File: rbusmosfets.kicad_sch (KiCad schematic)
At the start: 12 parts, among them J1 RBUS, J4 Conn_01x02_Male, Q4 PXP012-30QLJ, Q5 PXP012-30QLJ, Q6 PXP012-30QLJ, Q7 PXP012-30QLJ, U10 LTC4412xS6, U9 LTC4412xS6

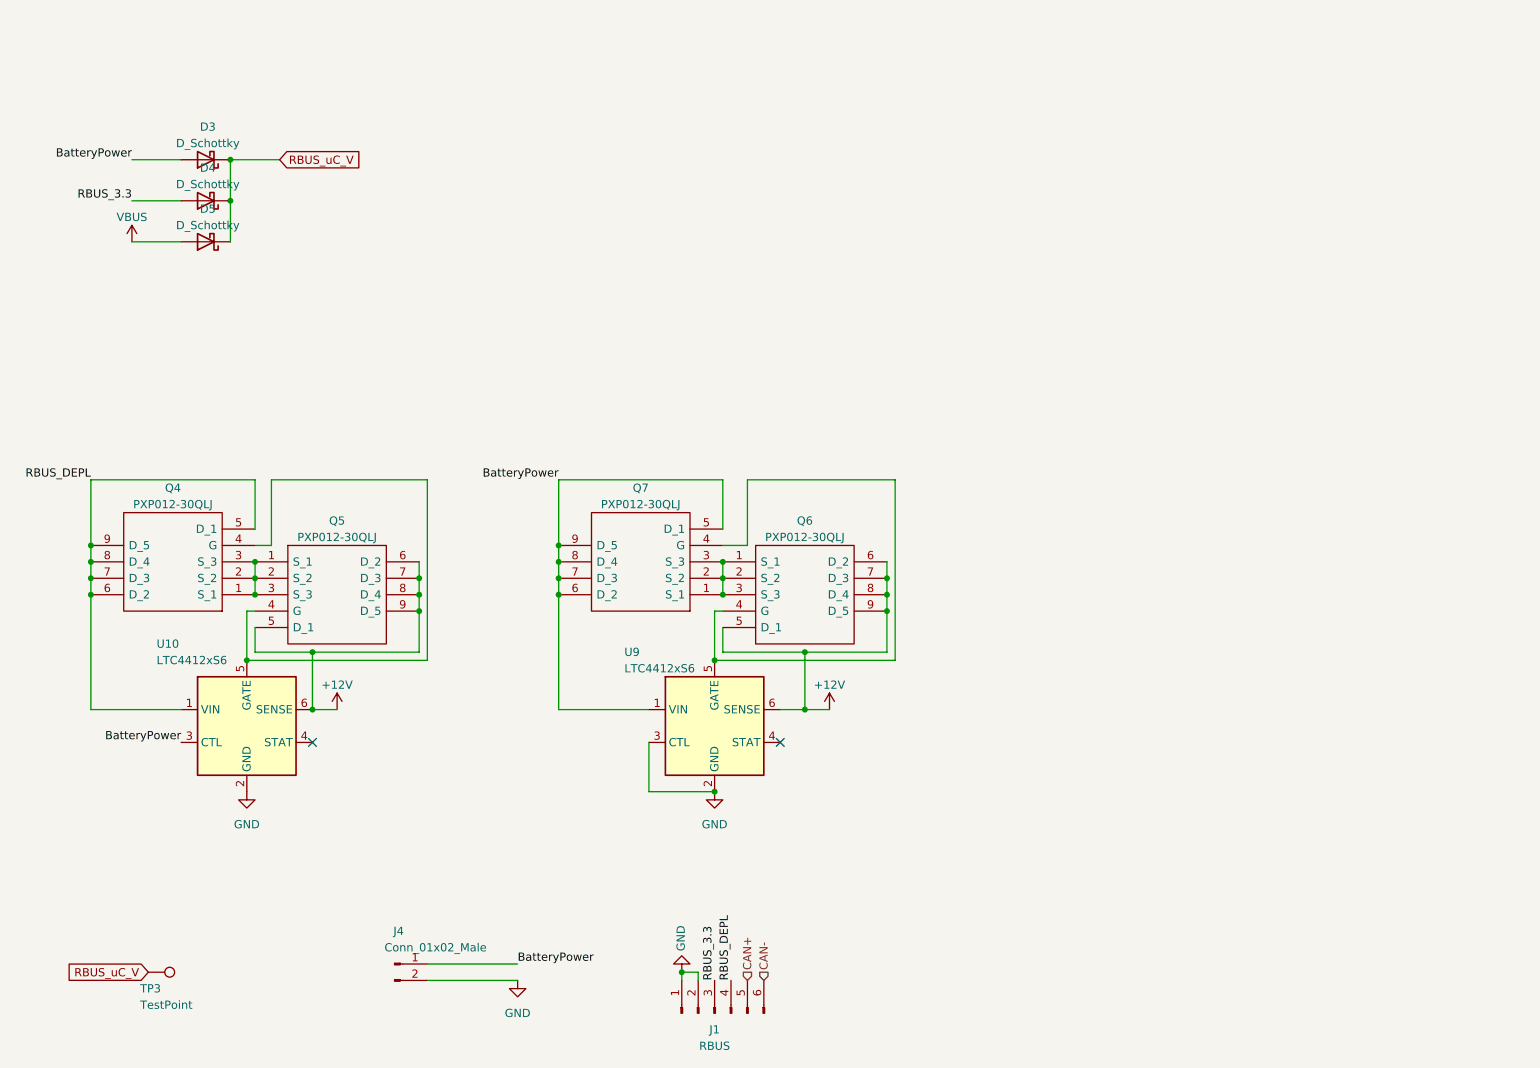
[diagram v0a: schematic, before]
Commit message: weird 3v3 and 3.3v bug
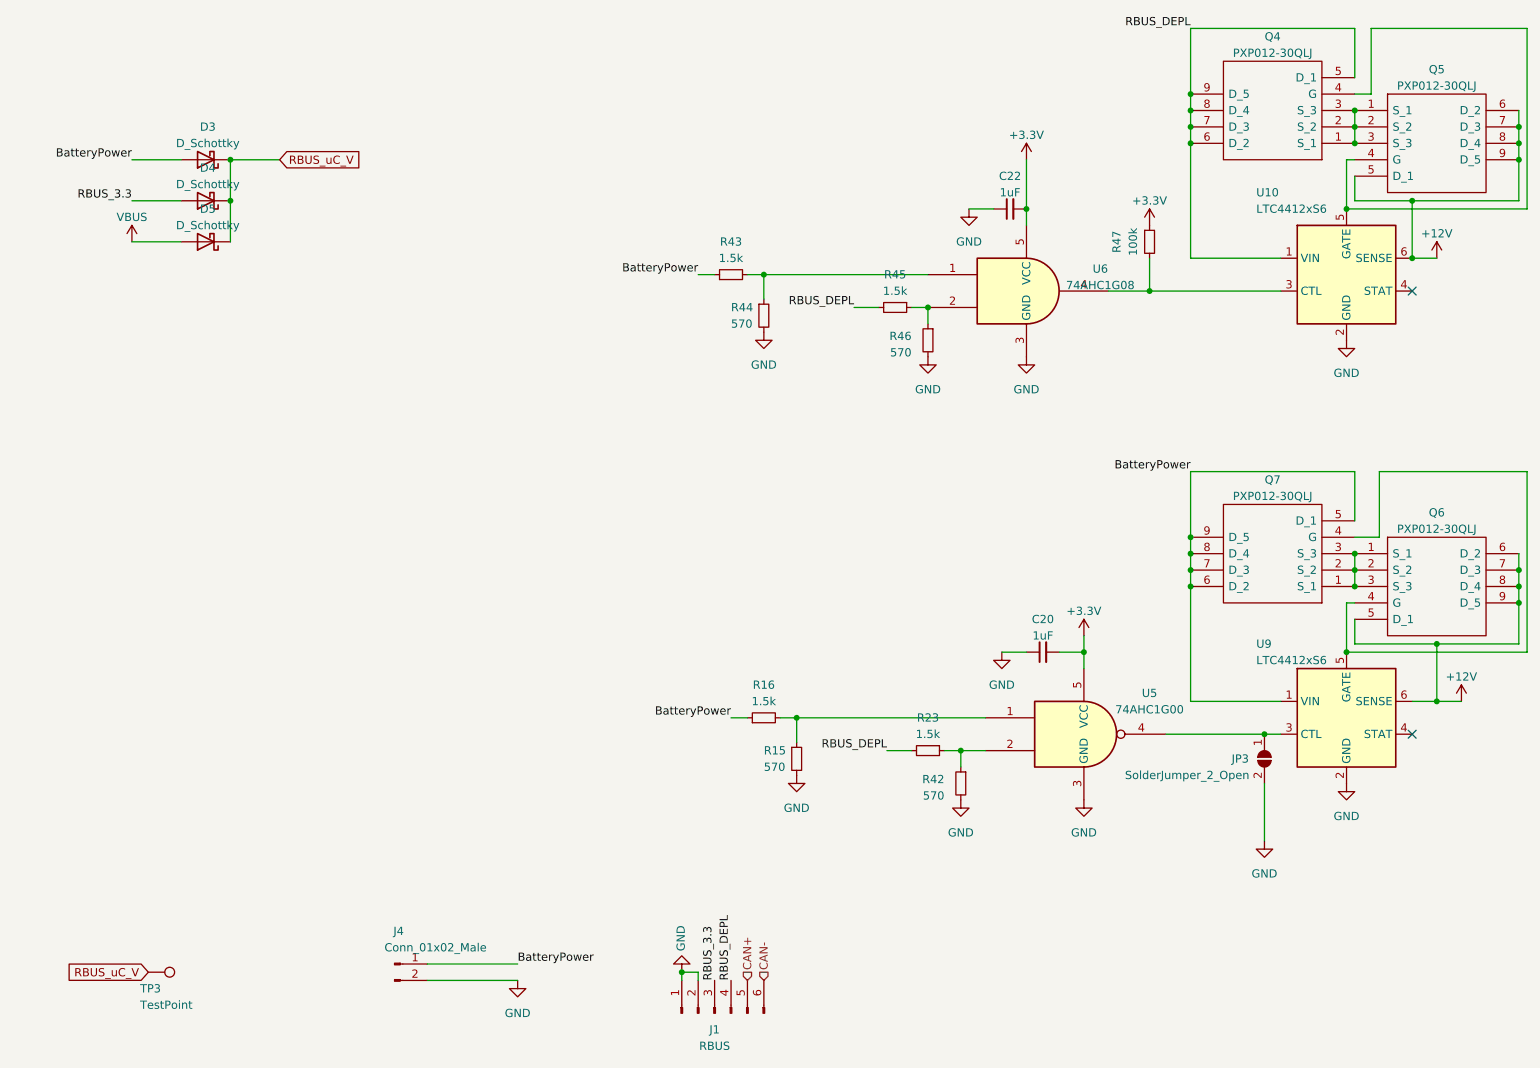
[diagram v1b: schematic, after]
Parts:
- added C20, C22: 1uF, Capacitor_SMD:C_0402_1005Metric, symbol Device:C_Small
- added JP3: SolderJumper_2_Open, Jumper:SolderJumper-2_P1.3mm_Open_RoundedPad1.0x1.5mm, symbol Jumper:SolderJumper_2_Open
- added R15, R42, R44, R46: 570, Resistor_SMD:R_0402_1005Metric, symbol Device:R_Small
- added R16, R23, R43, R45: 1.5k, Resistor_SMD:R_0402_1005Metric, symbol Device:R_Small
- added R47: 100k, Resistor_SMD:R_0402_1005Metric, symbol Device:R_Small
- added U5: 74AHC1G00, Package_TO_SOT_SMD:SOT-353_SC-70-5, symbol 74xGxx:74AHC1G00
- added U6: 74AHC1G08, Package_TO_SOT_SMD:SOT-353_SC-70-5, symbol 74xGxx:74AHC1G08
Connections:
- net BatteryPower: now also R16.1, R43.1; no longer U10.3 (CTL)
- net GND: now also C20.1, C22.1, JP3.2 (B), R15.2, R42.2, R44.2, R46.2, U5.3 (GND), U6.3 (GND); no longer U9.3 (CTL)
- net RBUS_DEPL: now also R23.2, R45.2
- new net: R43.2, R44.1, U6.1
- new net: R45.1, R46.1, U6.2
- new net: R47.2, U10.3 (CTL), U6.4
- new net: R15.1, R16.2, U5.1
- new net: R23.1, R42.1, U5.2
- new net: JP3.1 (A), U5.4, U9.3 (CTL)
- new net +3.3V: C20.2, C22.2, R47.1, U5.5 (VCC), U6.5 (VCC)
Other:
- moved on the sheet: Q4, Q5, Q6, Q7, U10, U9
